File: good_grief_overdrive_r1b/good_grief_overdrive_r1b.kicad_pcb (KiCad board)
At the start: 2 copper layers, 86.4 x 95.3 mm, 67 parts, among them J1 0.5, J2 0.5, X1 +, X2 -, X3 COM, X4 COM

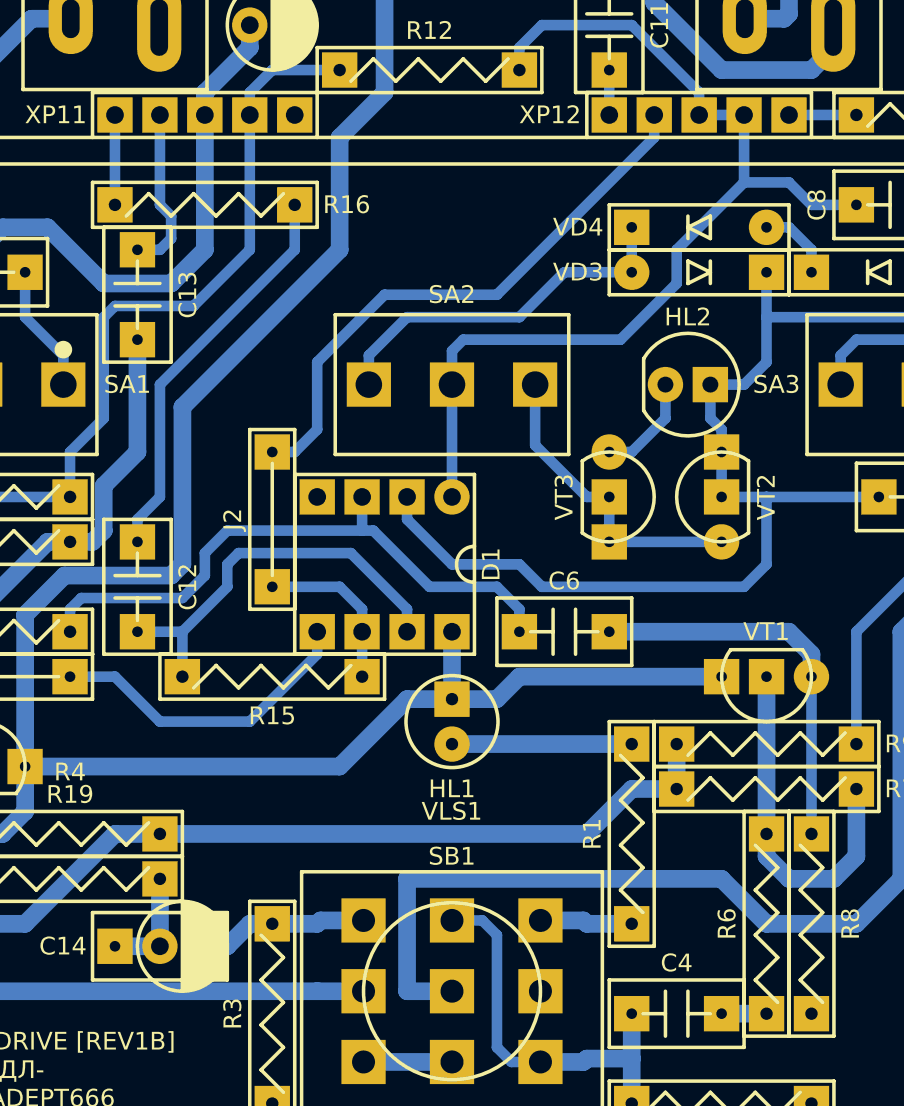
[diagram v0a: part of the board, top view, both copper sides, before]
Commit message: Good Grief Overdrive [REV1B]: minor changes
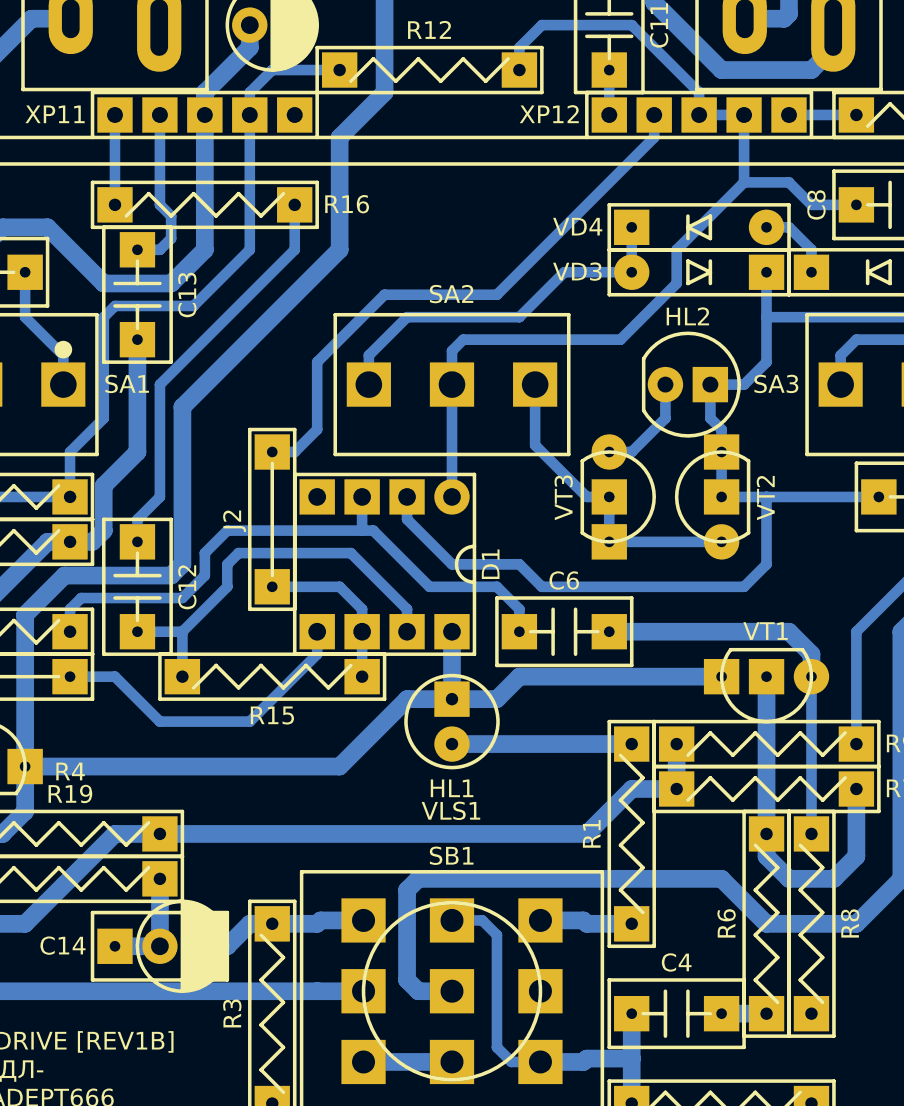
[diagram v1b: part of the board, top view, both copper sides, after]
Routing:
- net /IN-CON: track 114.8 -> 114.0 mm
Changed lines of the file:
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@@
     (thickness 1.5)
     (drawings 11)
-    (tracks 275)
+    (tracks 277)
     (zones 0)
     (modules 67)
@@
     (mod_text_size 1 1)
     (mod_text_width 0.15)
-    (pad_size 3 3)
-    (pad_drill 1.5)
+    (pad_size 2 2)
+    (pad_drill 0.9)
     (pad_to_mask_clearance 0.2)
     (solder_mask_min_width 0.1)
@@
       (effects (font (size 1 1) (thickness 0.2)))
     )
-    (fp_arc (start 1.27 0) (end -0.699999 1.499999) (angle -285.4271628) (layer F.Fab) (width 0.2))
-    (fp_arc (start 0.6 0) (end 0.6 1.5) (angle -180) (layer F.Fab) (width 0.2))
-    (fp_arc (start -0.6 0) (end -0.6 -1.5) (angle -180) (layer F.Fab) (width 0.2))
     (fp_line (start 1.27 -2.54) (end 1.27 2.54) (layer F.SilkS) (width 0.2))
     (fp_poly (pts (xy 3.81 1.905) (xy 3.048 1.905) (xy 2.159 2.413) (xy 1.27 2.54)
@@
     (fp_line (start 3.175 -1.905) (end 3.81 -1.905) (layer F.CrtYd) (width 0.1))
     (fp_line (start 3.175 1.905) (end 3.81 1.905) (layer F.CrtYd) (width 0.1))
+    (fp_arc (start 1.27 0) (end -0.699999 1.499999) (angle -285.4271628) (layer F.Fab) (width 0.2))
+    (fp_arc (start 0.6 0) (end 0.6 1.5) (angle -180) (layer F.Fab) (width 0.2))
+    (fp_arc (start -0.6 0) (end -0.6 -1.5) (angle -180) (layer F.Fab) (width 0.2))
     (pad - thru_hole rect (at 2.54 0) (size 2 2) (drill 1) (layers B.Cu B.Mask)
       (net 40 /OUT-CIR))
@@
       (effects (font (size 1 1) (thickness 0.2)) (justify right))
     )
-    (pad 22 thru_hole rect (at 8.89 11.23) (size 2 2) (drill 1) (layers B.Cu B.Mask)
+    (pad 22 thru_hole rect (at 8.89 11.23) (size 2 2) (drill 0.9) (layers B.Cu B.Mask)
       (net 29 "Net-(C11-Pad1)"))
-    (pad 23 thru_hole rect (at 11.43 11.23) (size 2 2) (drill 1) (layers B.Cu B.Mask)
+    (pad 23 thru_hole rect (at 11.43 11.23) (size 2 2) (drill 0.9) (layers B.Cu B.Mask)
       (net 38 /RP23))
-    (pad 33 thru_hole rect (at 13.97 11.23) (size 2 2) (drill 1) (layers B.Cu B.Mask)
+    (pad 33 thru_hole rect (at 13.97 11.23) (size 2 2) (drill 0.9) (layers B.Cu B.Mask)
       (net 26 "Net-(C8-Pad2)"))
-    (pad 32 thru_hole rect (at 16.51 11.23) (size 2 2) (drill 1) (layers B.Cu B.Mask)
+    (pad 32 thru_hole rect (at 16.51 11.23) (size 2 2) (drill 0.9) (layers B.Cu B.Mask)
       (net 26 "Net-(C8-Pad2)"))
-    (pad 31 thru_hole rect (at 19.05 11.23) (size 2 2) (drill 1) (layers B.Cu B.Mask)
+    (pad 31 thru_hole rect (at 19.05 11.23) (size 2 2) (drill 0.9) (layers B.Cu B.Mask)
       (net 20 "Net-(R11-Pad2)"))
-    (pad 22 thru_hole rect (at -8.89 11.23) (size 2 2) (drill 1) (layers B.Cu B.Mask)
+    (pad 22 thru_hole rect (at -8.89 11.23) (size 2 2) (drill 0.9) (layers B.Cu B.Mask)
       (net 29 "Net-(C11-Pad1)"))
-    (pad 12 thru_hole rect (at -16.51 11.23) (size 2 2) (drill 1) (layers B.Cu B.Mask)
+    (pad 12 thru_hole rect (at -16.51 11.23) (size 2 2) (drill 0.9) (layers B.Cu B.Mask)
       (net 33 "Net-(C13-Pad1)"))
-    (pad 11 thru_hole rect (at -13.97 11.23) (size 2 2) (drill 1) (layers B.Cu B.Mask)
+    (pad 11 thru_hole rect (at -13.97 11.23) (size 2 2) (drill 0.9) (layers B.Cu B.Mask)
       (net 36 VREF))
-    (pad 13 thru_hole rect (at -19.05 11.23) (size 2 2) (drill 1) (layers B.Cu B.Mask)
+    (pad 13 thru_hole rect (at -19.05 11.23) (size 2 2) (drill 0.9) (layers B.Cu B.Mask)
       (net 15 "Net-(R16-Pad2)"))
-    (pad 21 thru_hole rect (at -11.43 11.23) (size 2 2) (drill 1) (layers B.Cu B.Mask)
+    (pad 21 thru_hole rect (at -11.43 11.23) (size 2 2) (drill 0.9) (layers B.Cu B.Mask)
       (net 37 /RP21))
   )
@@
   (segment (start 123.19 173.99) (end 128.27 173.99) (width 1) (layer B.Cu) (net 5))
   (segment (start 120.65 171.45) (end 123.19 173.99) (width 1) (layer B.Cu) (net 5))
-  (segment (start 102.87 171.45) (end 120.65 171.45) (width 1) (layer B.Cu) (net 5))
-  (segment (start 102.87 177.8) (end 102.87 171.45) (width 1) (layer B.Cu) (net 5))
   (segment (start 139.7 139.7) (end 140.97 138.43) (width 1) (layer B.Cu) (net 5))
   (segment (start 140.97 138.43) (end 140.97 127) (width 1) (layer B.Cu) (net 5))
-  (segment (start 105.41 177.8) (end 102.87 177.8) (width 1) (layer B.Cu) (net 5))
   (segment (start 138.43 147.32) (end 139.7 146.05) (width 1) (layer B.Cu) (net 5))
   (segment (start 139.7 146.05) (end 139.7 139.7) (width 1) (layer B.Cu) (net 5))
@@
   (segment (start 124.185 122.83) (end 124.46 122.555) (width 1) (layer B.Cu) (net 5))
   (segment (start 121.96 122.83) (end 124.185 122.83) (width 1) (layer B.Cu) (net 5))
+  (segment (start 103.505 171.45) (end 120.65 171.45) (width 1) (layer B.Cu) (net 5))
+  (segment (start 102.87 172.085) (end 103.505 171.45) (width 1) (layer B.Cu) (net 5))
+  (segment (start 102.87 177.165) (end 103.505 177.8) (width 1) (layer B.Cu) (net 5))
+  (segment (start 105.41 177.8) (end 103.505 177.8) (width 1) (layer B.Cu) (net 5))
+  (segment (start 102.87 177.165) (end 102.87 172.085) (width 1) (layer B.Cu) (net 5))
   (segment (start 97.79 177.8) (end 100.41 177.8) (width 1) (layer B.Cu) (net 6))
   (segment (start 74.93 177.8) (end 97.79 177.8) (width 1) (layer B.Cu) (net 6))
@@
   (segment (start 81.28 173.99) (end 86.36 168.91) (width 1) (layer B.Cu) (net 36))
   (segment (start 76.2 173.99) (end 81.28 173.99) (width 1) (layer B.Cu) (net 36))
+  (segment (start 88.9 168.91) (end 113.03 168.91) (width 1) (layer B.Cu) (net 36))
+  (segment (start 113.03 168.91) (end 115.57 166.37) (width 1) (layer B.Cu) (net 36))
   (segment (start 115.57 166.37) (end 118.11 166.37) (width 1) (layer B.Cu) (net 36))
-  (segment (start 113.03 168.91) (end 115.57 166.37) (width 1) (layer B.Cu) (net 36))
-  (segment (start 88.9 168.91) (end 113.03 168.91) (width 1) (layer B.Cu) (net 36))
   (segment (start 78.74 143.51) (end 78.74 149.86) (width 0.6) (layer B.Cu) (net 37))
   (segment (start 76.2 152.4) (end 76.2 160.02) (width 0.6) (layer B.Cu) (net 37))
